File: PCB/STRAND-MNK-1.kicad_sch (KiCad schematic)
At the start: 43 parts

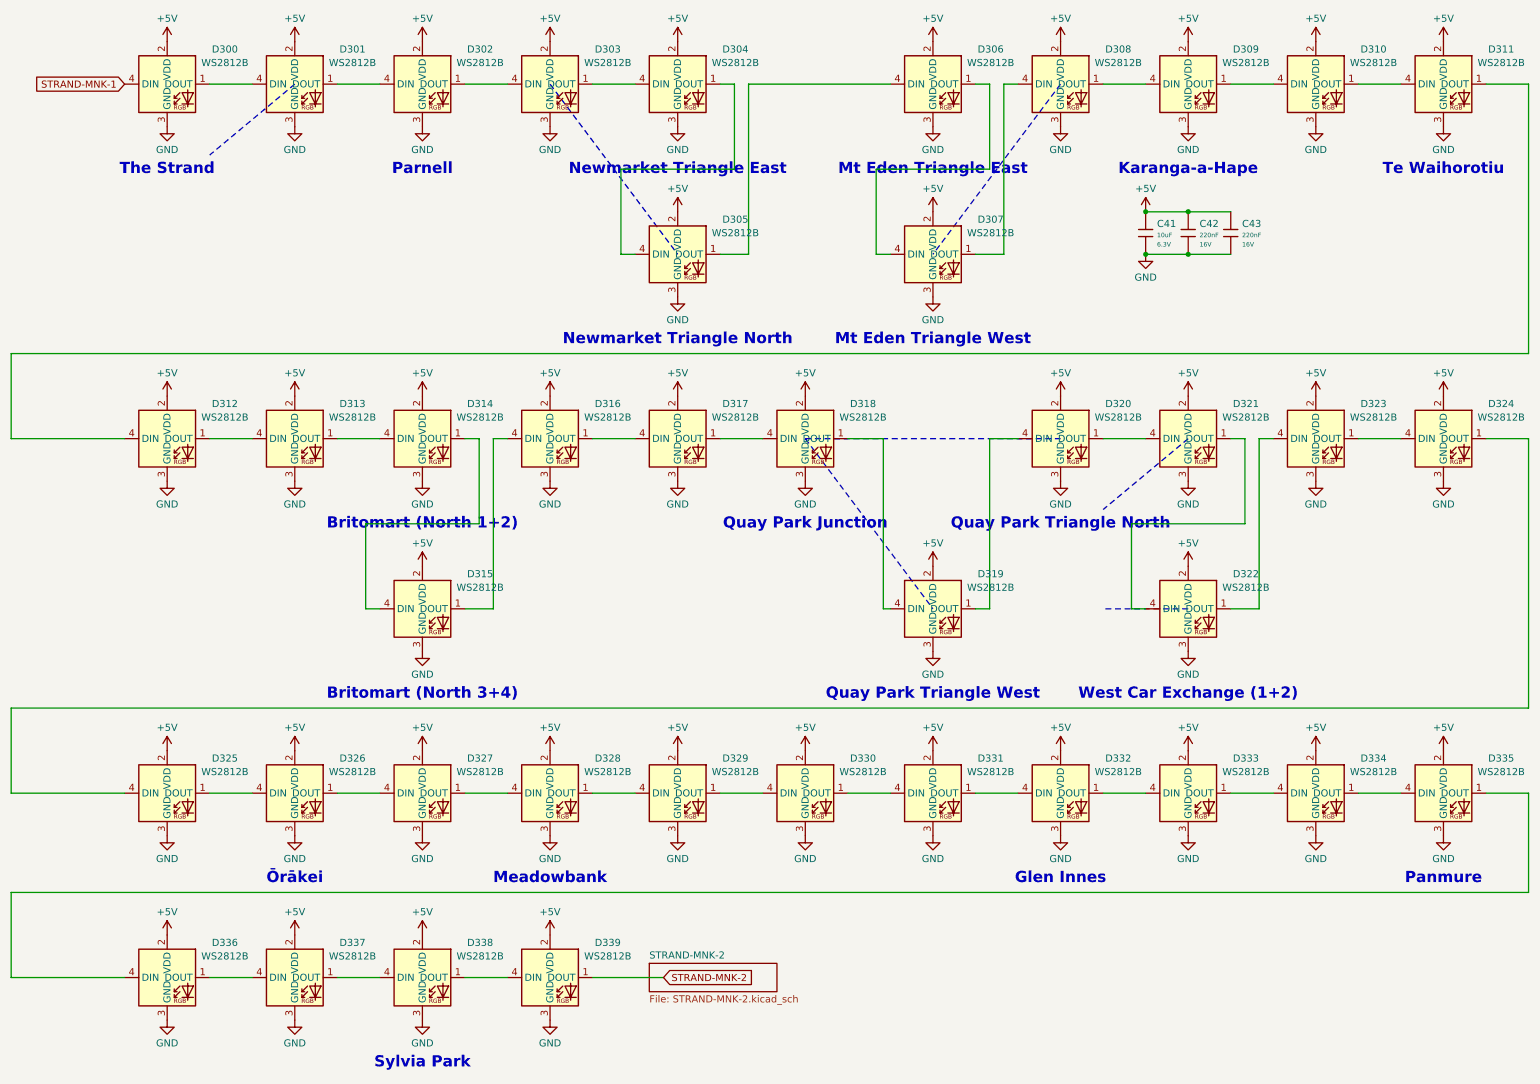
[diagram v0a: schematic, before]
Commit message: Final tweaks for V1.0.0
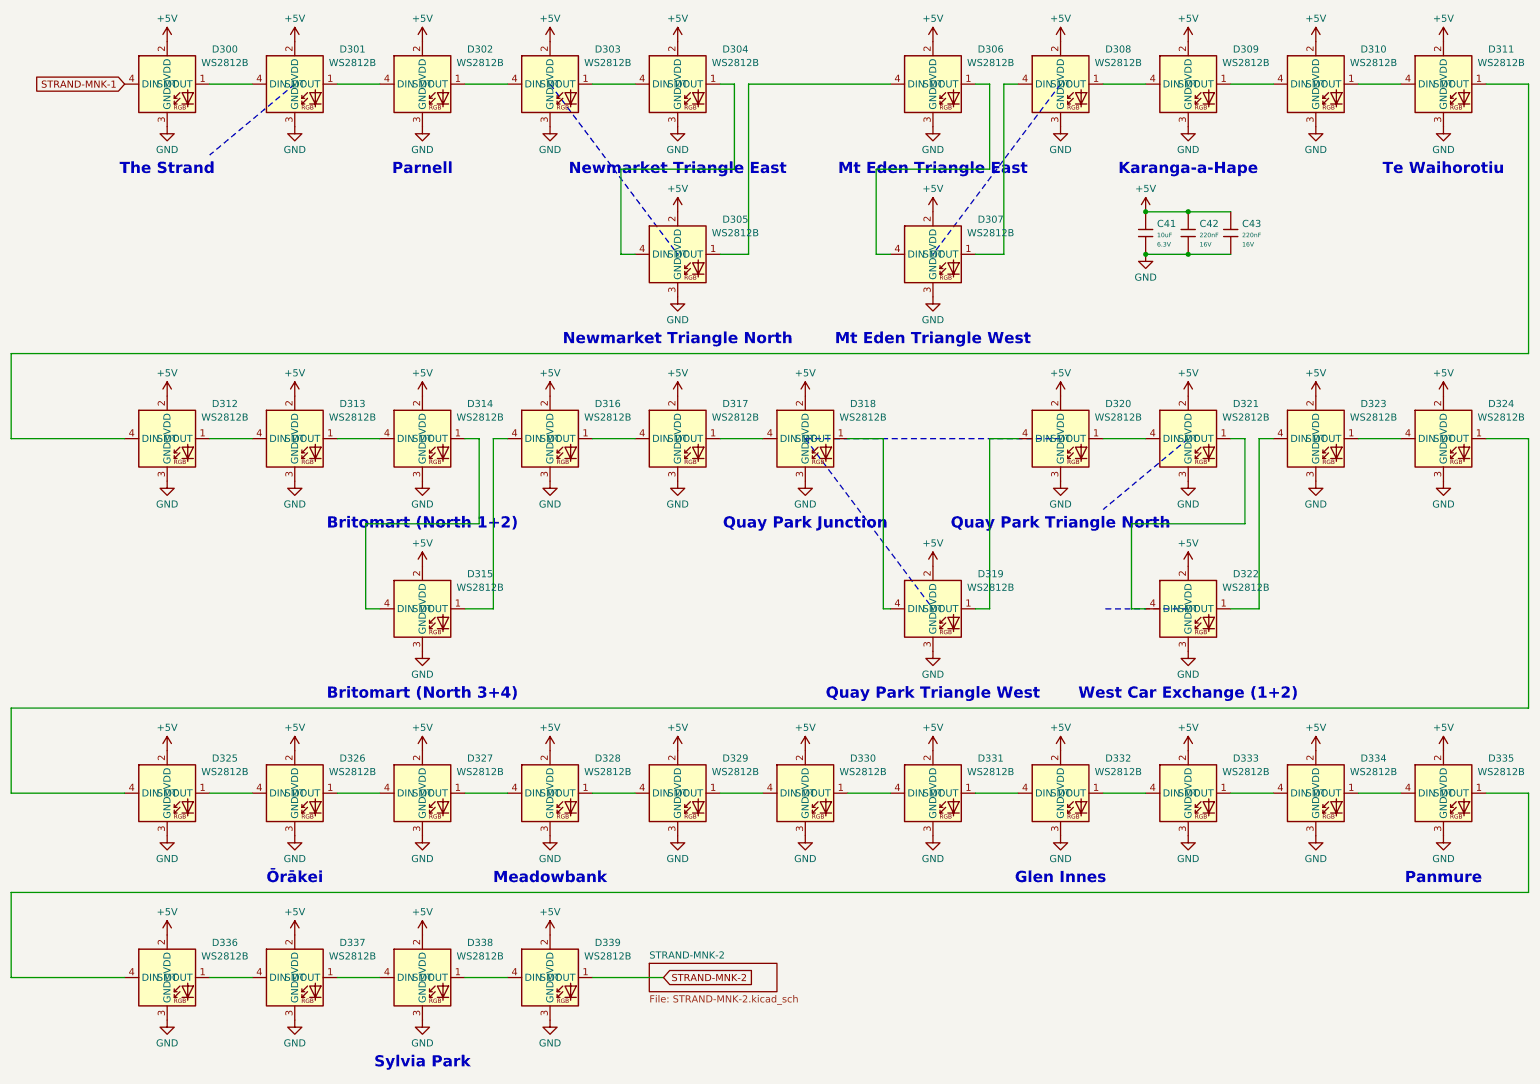
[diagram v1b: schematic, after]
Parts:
- D300, D301, D302, D303, D304, D305, D306, D307, D308, D309, D310, D311, D312, D313, D314, D315, D316, D317, D318, D319, D320, D321, D322, D323, D324, D325, D326, D327, D328, D329, D330, D331, D332, D333, D334, D335, D336, D337, D338, D339: Manufacturer (none) -> XINGLIGHT; Part (none) -> XL-1615RGBC-WS2812B; Process (none) -> SMT
